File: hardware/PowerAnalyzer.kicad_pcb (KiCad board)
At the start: 2 copper layers, 53.4 x 45.7 mm, 68 parts, among them J1 EXPANSION, J10 TEST_IN, J11 PWR_IN, J12 PWR_OUT, J2 UDPI, J3 I2C, J4 FAN_OUT, J5 NTC, J6 UART, J7 USB_C_Receptacle_USB2.0_16P, J8 FAN_IN, Q1 SI2302, Q2 IRL540NPBF, U1 ATTINY814-SSN, U2 FT230XS, U3 INA219, U4 LMV321, U5 INA219

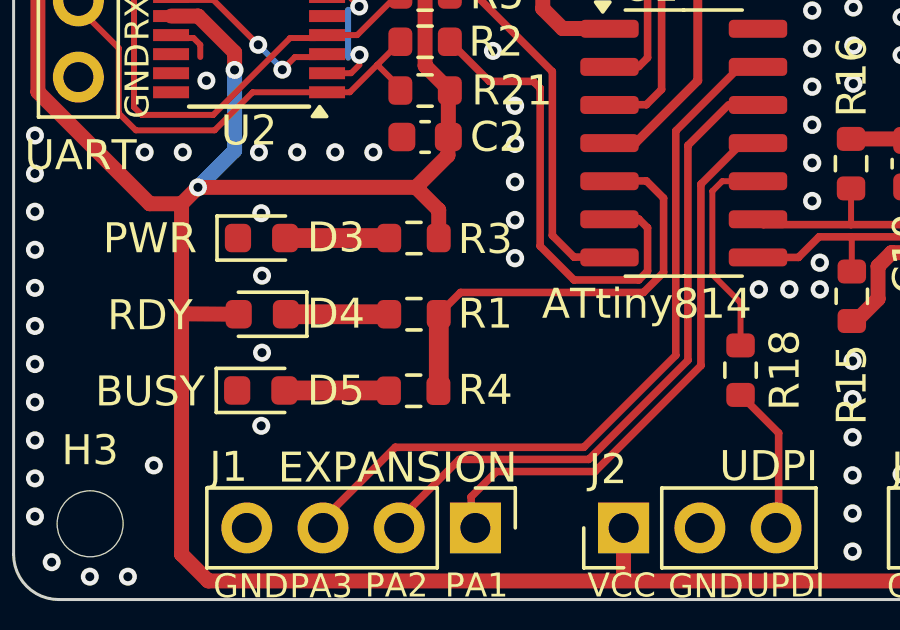
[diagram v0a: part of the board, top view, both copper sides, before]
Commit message: Finish (?) KiCadifying
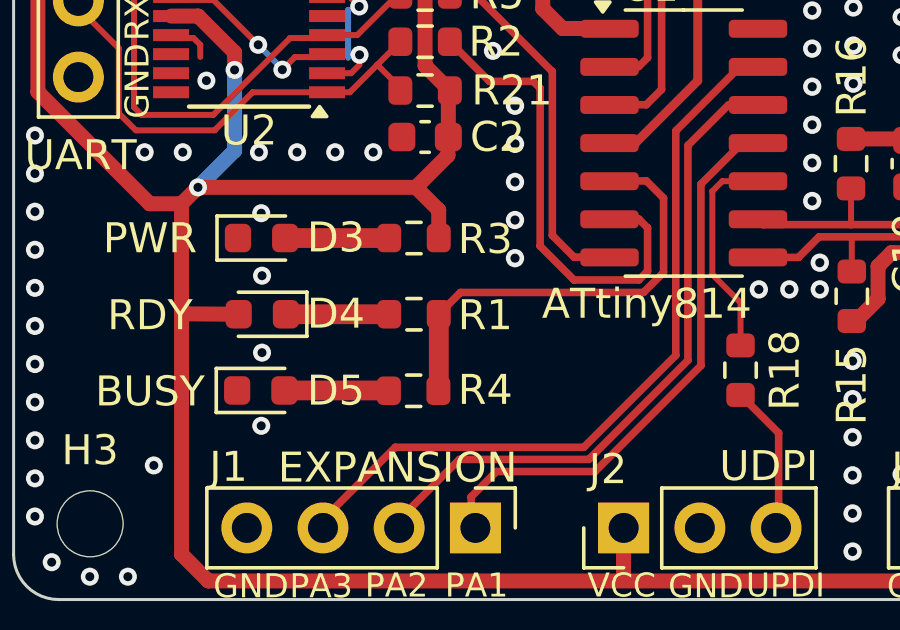
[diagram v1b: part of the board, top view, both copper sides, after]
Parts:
- turned R1 to 0 degrees
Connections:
- R1 pad 1: LED -> Net-(D4-K)
- R1 pad 2: Net-(D4-K) -> LED
